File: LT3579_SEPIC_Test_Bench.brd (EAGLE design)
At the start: 84.9 x 63.2 mm, 160 parts

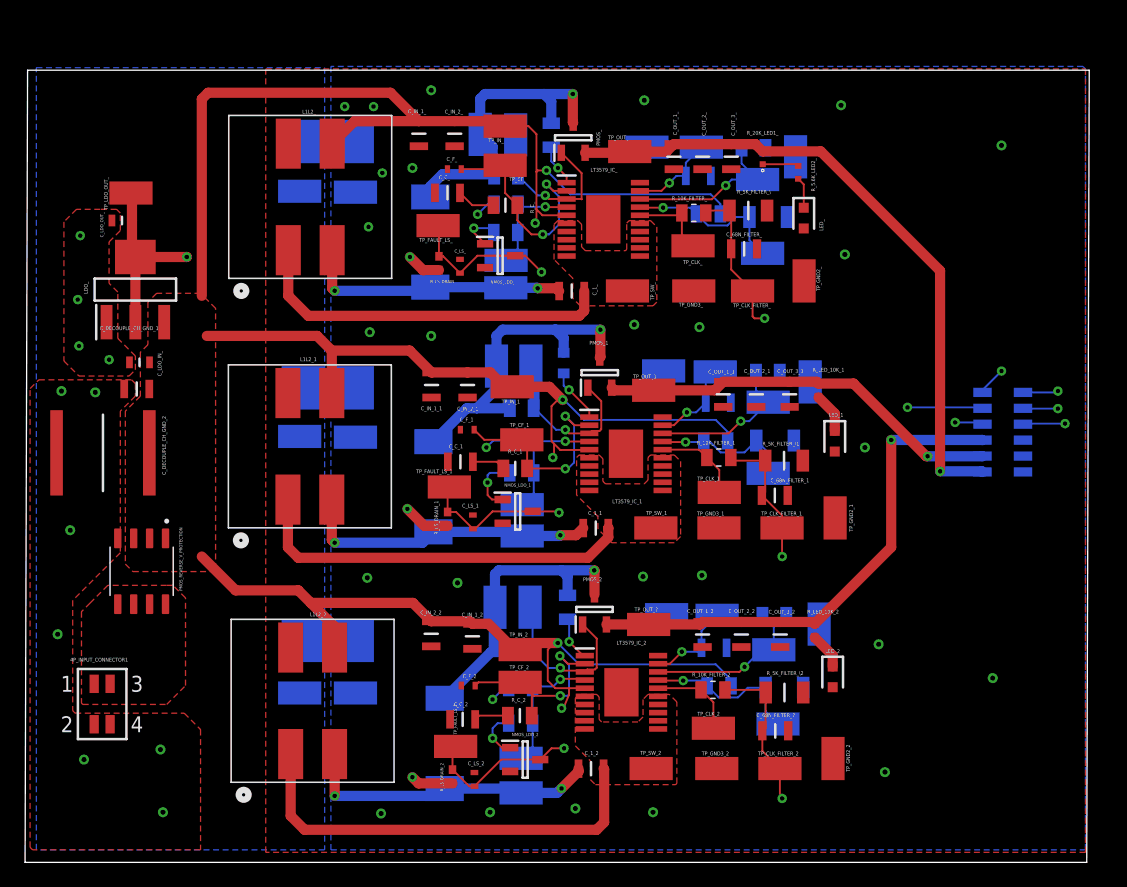
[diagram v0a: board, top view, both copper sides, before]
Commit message: modified routing
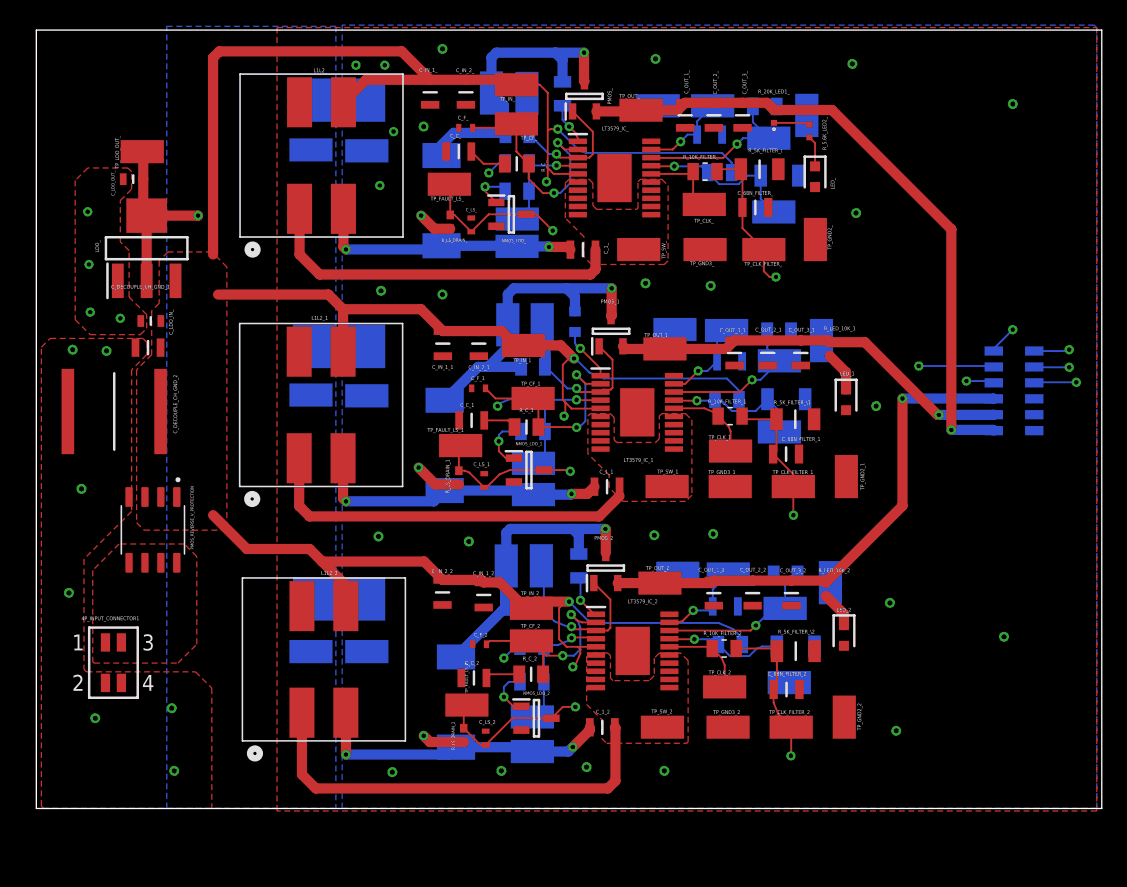
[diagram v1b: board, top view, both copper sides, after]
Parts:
- moved C_LS_ 3.42 mm to (34.7, 47.6)
- moved C_OUT_1_1 3.42 mm to (55.7, 37.3)
- moved TP_SHDN_ 3.42 mm to (58.8, 48.6)
- moved TP_SW_ 3.42 mm to (48.1, 45.6)
- moved C_DECOUPLE_CH_GND_1 3.42 mm to (8.91, 37.8)
- moved C_LDO_OUT_ 3.42 mm to (7.73, 51.2)
- moved C_68N_FILTER_ 3.42 mm to (57.4, 49.0)
- moved C_F_ 3.42 mm to (34.2, 55.3)
- moved C_F_1 3.42 mm to (35.3, 34.5)
- moved C_IN_1_1 3.42 mm to (32.4, 38.1)
- moved C_IN_2_1 3.42 mm to (35.3, 38.1)
- moved C_OUT_2_1 3.42 mm to (58.3, 37.3)
- moved C_OUT_3_1 3.42 mm to (61.0, 37.3)
- moved C_SS_1 3.42 mm to (55.3, 36.7)
- moved D1_ 3.42 mm to (32.3, 49.5)
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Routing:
- net VIN: track 219.3 -> 216.7 mm
- net SW1-2_1: track 31.1 -> 30.4 mm
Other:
- board size 84.9 x 63.2 mm -> 85 x 62.1 mm
